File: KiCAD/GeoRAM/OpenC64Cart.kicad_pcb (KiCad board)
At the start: 2 copper layers, 94.7 x 58.4 mm, 10 parts, among them U1 74HC04, U2 74LS08, U3 74LS00, U4 74LS573, U5 74LS573, U6 74HC245, U7 C64-Exp-Port

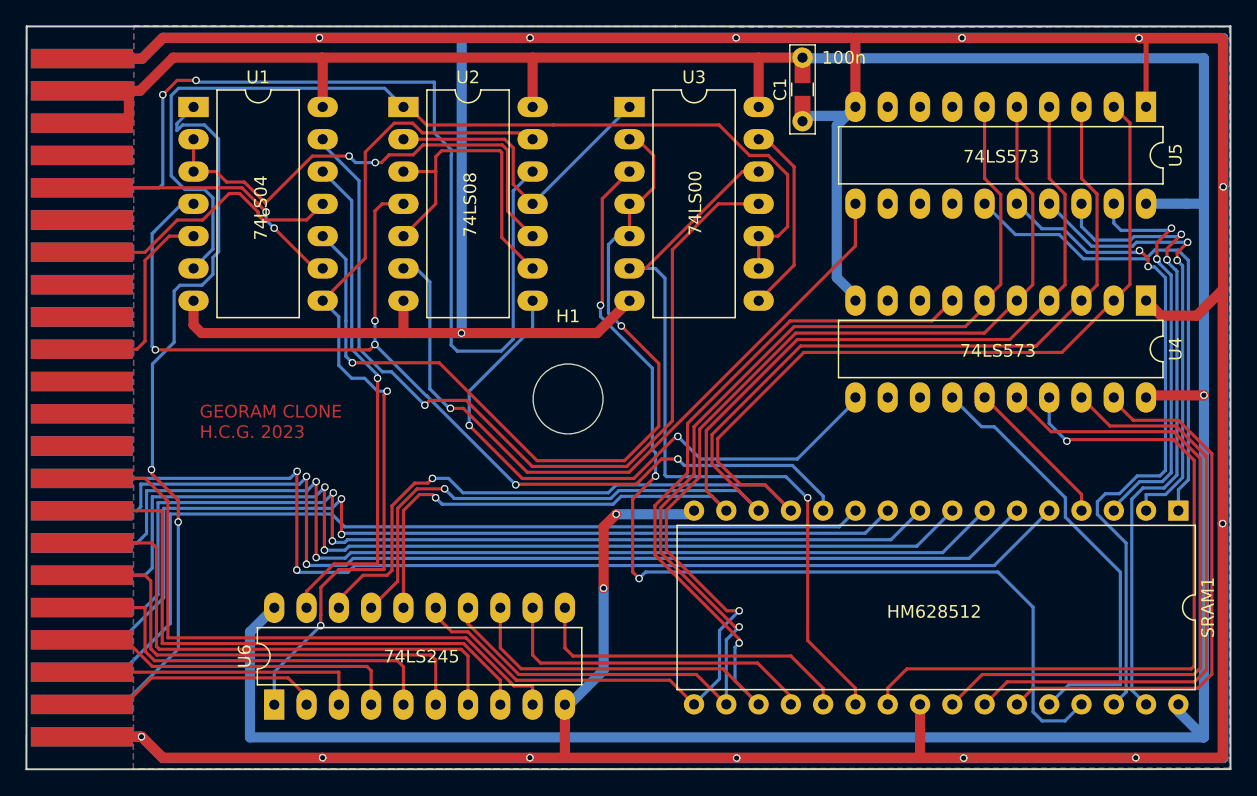
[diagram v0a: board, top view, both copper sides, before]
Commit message: Version 2.0, fixed several issues with the original design
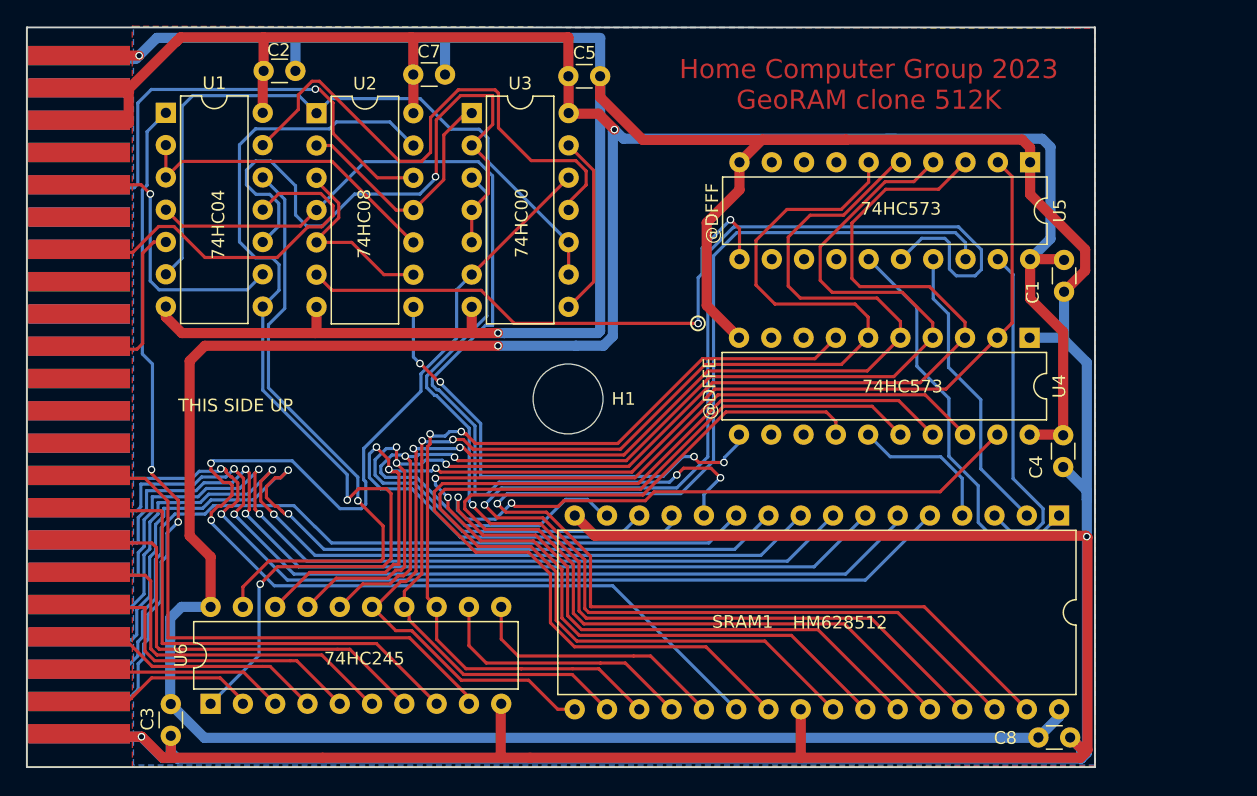
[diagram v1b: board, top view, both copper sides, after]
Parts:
- added C1: 100n, Capacitor_THT:C_Disc_D3.0mm_W1.6mm_P2.50mm, F.Cu at (184.9, 80.4)
- added C2: 100n, Capacitor_THT:C_Disc_D3.0mm_W1.6mm_P2.50mm, F.Cu at (124.4, 63.1)
- added C3: 100n, Capacitor_THT:C_Disc_D3.0mm_W1.6mm_P2.50mm, F.Cu at (114.6, 115.4)
- added C4: 100n, Capacitor_THT:C_Disc_D3.0mm_W1.6mm_P2.50mm, F.Cu at (184.8, 94.2)
- added C5: 100n, Capacitor_THT:C_Disc_D3.0mm_W1.6mm_P2.50mm, F.Cu at (148.4, 63.5)
- added C8: 100n, Capacitor_THT:C_Disc_D3.0mm_W1.6mm_P2.50mm, F.Cu at (185.3, 115.5)
- C7: renamed from C1; footprint OpenC64Cart:C_0805+THT -> Capacitor_THT:C_Disc_D3.0mm_W1.6mm_P2.50mm
- U1: value 74HC04 -> 7404; footprint Package_DIP:DIP-14_W10.16mm_LongPads -> Package_DIP:DIP-14_W7.62mm
- U2: value 74LS08 -> 7408; footprint Package_DIP:DIP-14_W10.16mm_LongPads -> Package_DIP:DIP-14_W7.62mm
- U3: value 74LS00 -> 7400; footprint Package_DIP:DIP-14_W10.16mm_LongPads -> Package_DIP:DIP-14_W7.62mm
- U4, U5, U6: footprint Package_DIP:DIP-20_W7.62mm_LongPads -> Package_DIP:DIP-20_W7.62mm
- moved C7 28.1 mm to (136.2, 63.4), turned to 180 degrees
- moved U3 12.4 mm to (138.3, 66.4)
- moved U5 10.1 mm to (182.2, 70.3)
- moved U4 9.61 mm to (182.2, 84.1)
- moved SRAM1 9.39 mm to (184.5, 98.0)
- moved U2 6.86 mm to (126.1, 66.4)
- moved U6 5.01 mm to (117.7, 112.8)
- moved U1 2.23 mm to (114.2, 66.4)
- moved U7 0.31 mm to (103.5, 59.3)
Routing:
- net GND: track 608.2 -> 466.9 mm, vias 16 -> 4
- net /A17: track 53.4 -> 118.5 mm, vias 2 -> 1
- net /A15: track 51.0 -> 107.4 mm, vias 2 -> 1
- net /A8: track 43.4 -> 91.1 mm, vias 0 -> 2
- net /A13: track 34.9 -> 79.4 mm
- net /A9: track 47.1 -> 90.1 mm, vias 0 -> 2
- net PHI: track 75.9 -> 37.3 mm, vias 2 -> 1
- net ~{CS} SRAM: track 61.6 -> 100.2 mm, vias 1 -> 2
- net +5V: track 259.5 -> 287.1 mm, vias 1 -> 2
- net /A11: track 53.6 -> 80.8 mm
- net Net-(U1-Pad13): track 69.7 -> 42.6 mm, vias 1 -> 0
- net /D1: track 96.1 -> 121.2 mm, vias 1 -> 3
- net /A10: track 57.0 -> 79.8 mm, vias 1 -> 0
- net Net-(U1-Pad6): track 76.0 -> 53.8 mm
- net /D2: track 89.0 -> 110.7 mm, vias 1 -> 2
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- added copper zone on B.Cu, net (none)
- added copper zone on F.Cu, net (none)
- removed copper zone on B.Cu, net GND
- removed copper zone on F.Cu, net GND
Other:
- board size 94.7 x 58.4 mm -> 84 x 58.2 mm
- board text added: "74HC00"
- board text added: "74HC04"
- board text added: "74HC08"
- board text added: "74HC245"
- board text added: "74HC573"
- board text added: "@DFFE"
- board text added: "@DFFF"
- board text added: "Home Computer Group 2023 GeoRAM clone 512K"
- board text added: "THIS SIDE UP"
- board text removed: "100n"
- board text removed: "74LS00"
- board text removed: "74LS04"
- board text removed: "74LS08"
- board text removed: "74LS245"
- board text removed: "74LS573"
- board text removed: "GEORAM CLONE H.C.G. 2023"
